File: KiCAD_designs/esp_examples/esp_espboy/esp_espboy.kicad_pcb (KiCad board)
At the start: 2 copper layers, 57 x 72 mm, 26 parts, among them J1 B4B-ZR-SM4-TFT_LF__SN_, J2 B2B-PH-SM4-TBLFSN, J3 Conn_01x02_Pin, J4 B4B-ZR-SM4-TFT_LF__SN_, J5 Conn_01x02_Pin, J6 B7B-ZR-SM4-TFT_LF__SN_, SW2 RS-282G05A3-SM RT, SW3 RS-282G05A3-SM RT, U1 ESP-12F, U2 AMS1117-3.3, U3 MCP23017-E_SO

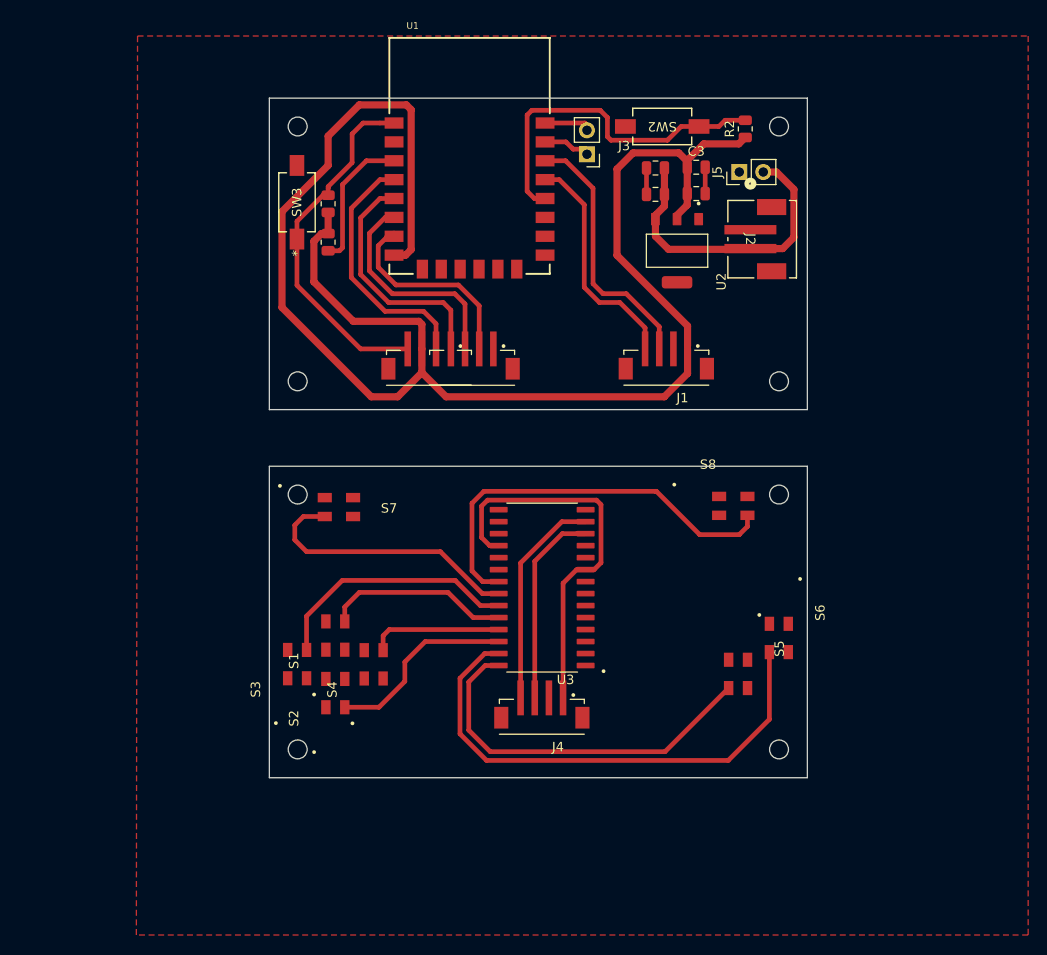
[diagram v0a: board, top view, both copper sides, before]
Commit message: larger button boy
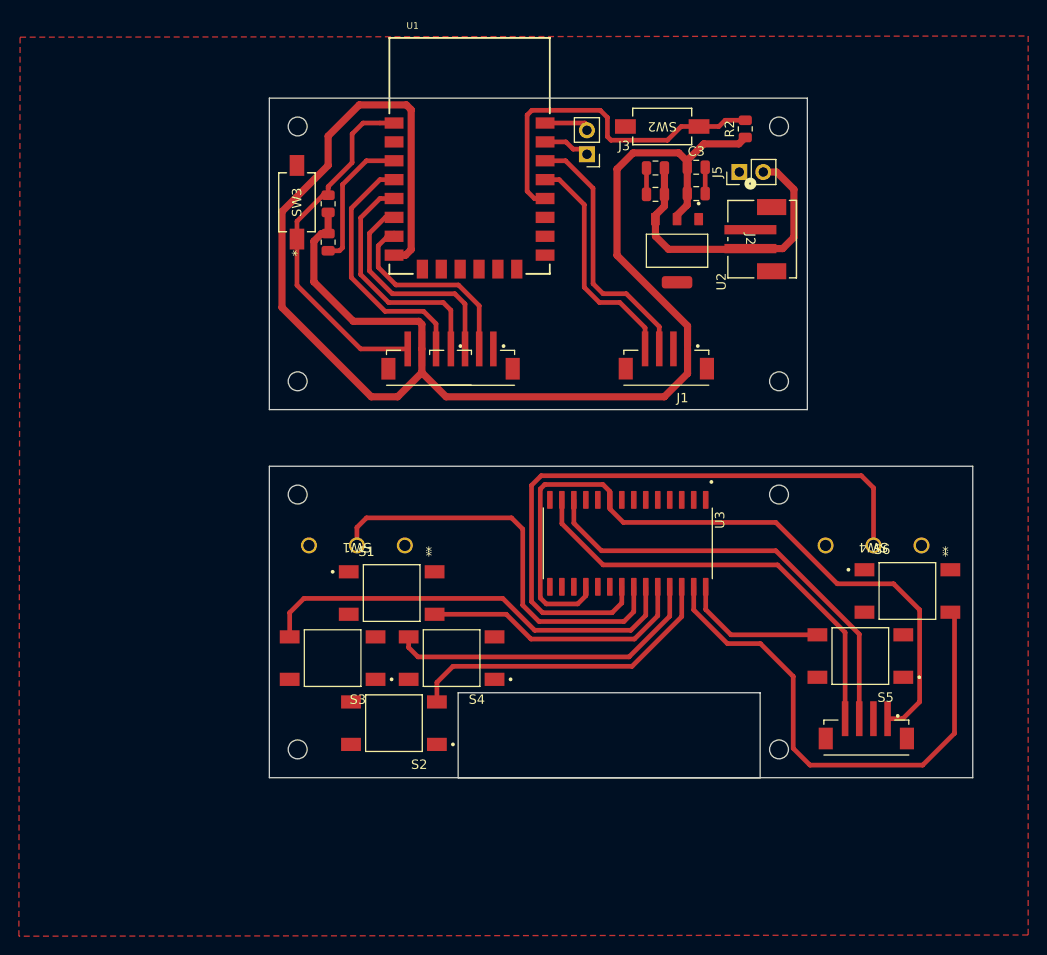
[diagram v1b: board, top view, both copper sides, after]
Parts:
- removed S7: RL, esp_lib:switch
- removed S8: RR, esp_lib:switch
- added SW1: D2FS-FL-N-A, esp_lib:D2FS-FL-N-A_OMR, F.Cu at (54.4, 72.4)
- added SW4: D2FS-FL-N-A, esp_lib:D2FS-FL-N-A_OMR, F.Cu at (109.1, 72.4)
- S1, S2, S3, S4, S5, S6: footprint esp_lib:switch -> esp_lib:switch_6
- moved J4 34.5 mm to (103.3, 92.7)
- moved S6 14.5 mm to (107.6, 77.2), turned to 0 degrees
- moved S5 13.1 mm to (102.6, 84.1), turned to 180 degrees
- moved U3 10.2 mm to (78.0, 72.2), turned to -90 degrees
- moved S4 8.28 mm to (59.3, 84.3), turned to 180 degrees
- moved S1 7.48 mm to (53.0, 77.4), turned to 0 degrees
- moved S2 6.98 mm to (53.2, 91.2), turned to 180 degrees
- moved S3 3.81 mm to (46.7, 84.3), turned to 180 degrees
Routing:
- net VCC: track 213.8 -> 250.7 mm
- net /SCK_mcp: track 49.6 -> 75.1 mm
- net /A: track 40.3 -> 15.3 mm
- net /RR: track 43.6 -> 67.8 mm
- net /SDA_mcp: track 47.8 -> 71.2 mm
- net /right: track 14.0 -> 34.1 mm
- net /left: track 26.6 -> 46.0 mm
- net /RL: track 29.1 -> 44.0 mm
- net /down: track 20.4 -> 34.1 mm
- net /up: track 19.6 -> 28.8 mm
- net /B: track 53.9 -> 55.7 mm
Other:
- board size 57 x 72 mm -> 74.5 x 72 mm
